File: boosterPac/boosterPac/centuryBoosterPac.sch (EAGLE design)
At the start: 5 parts, among them J1 22-05-7028-02, J2 22-05-7028-02, Q1 BSS123

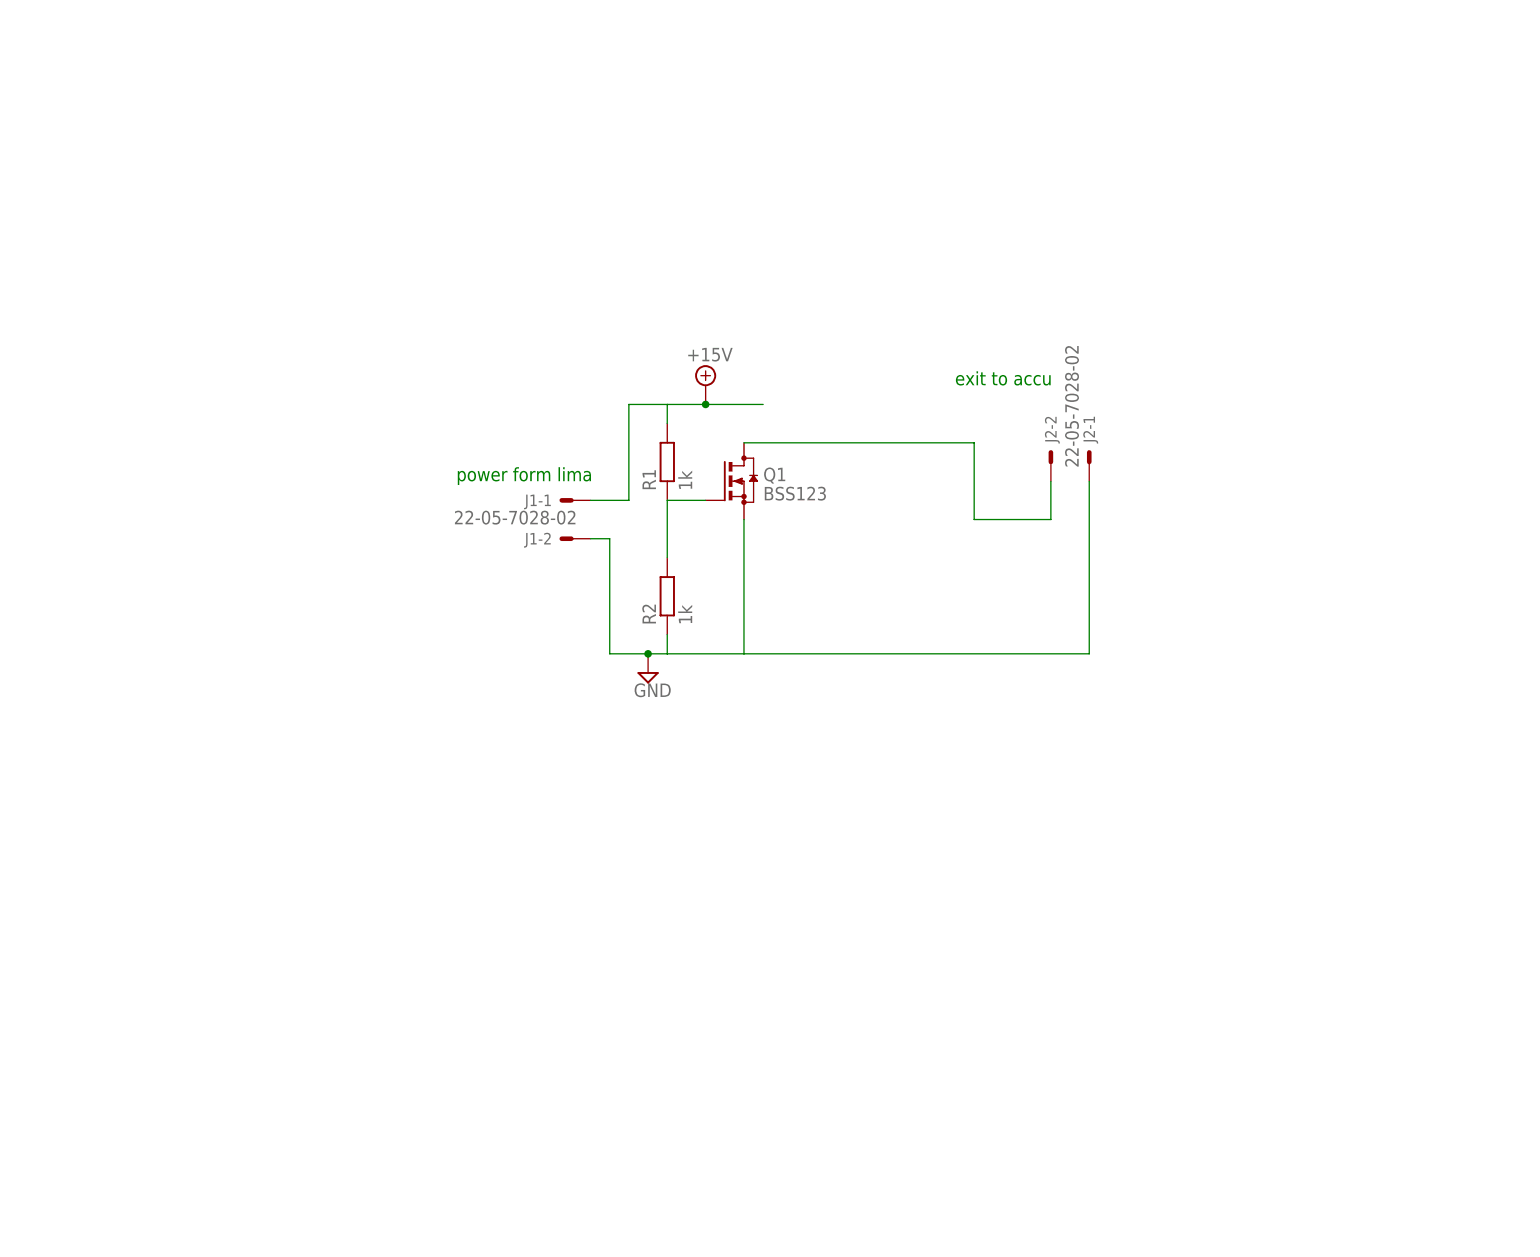
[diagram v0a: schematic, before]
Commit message: reg save
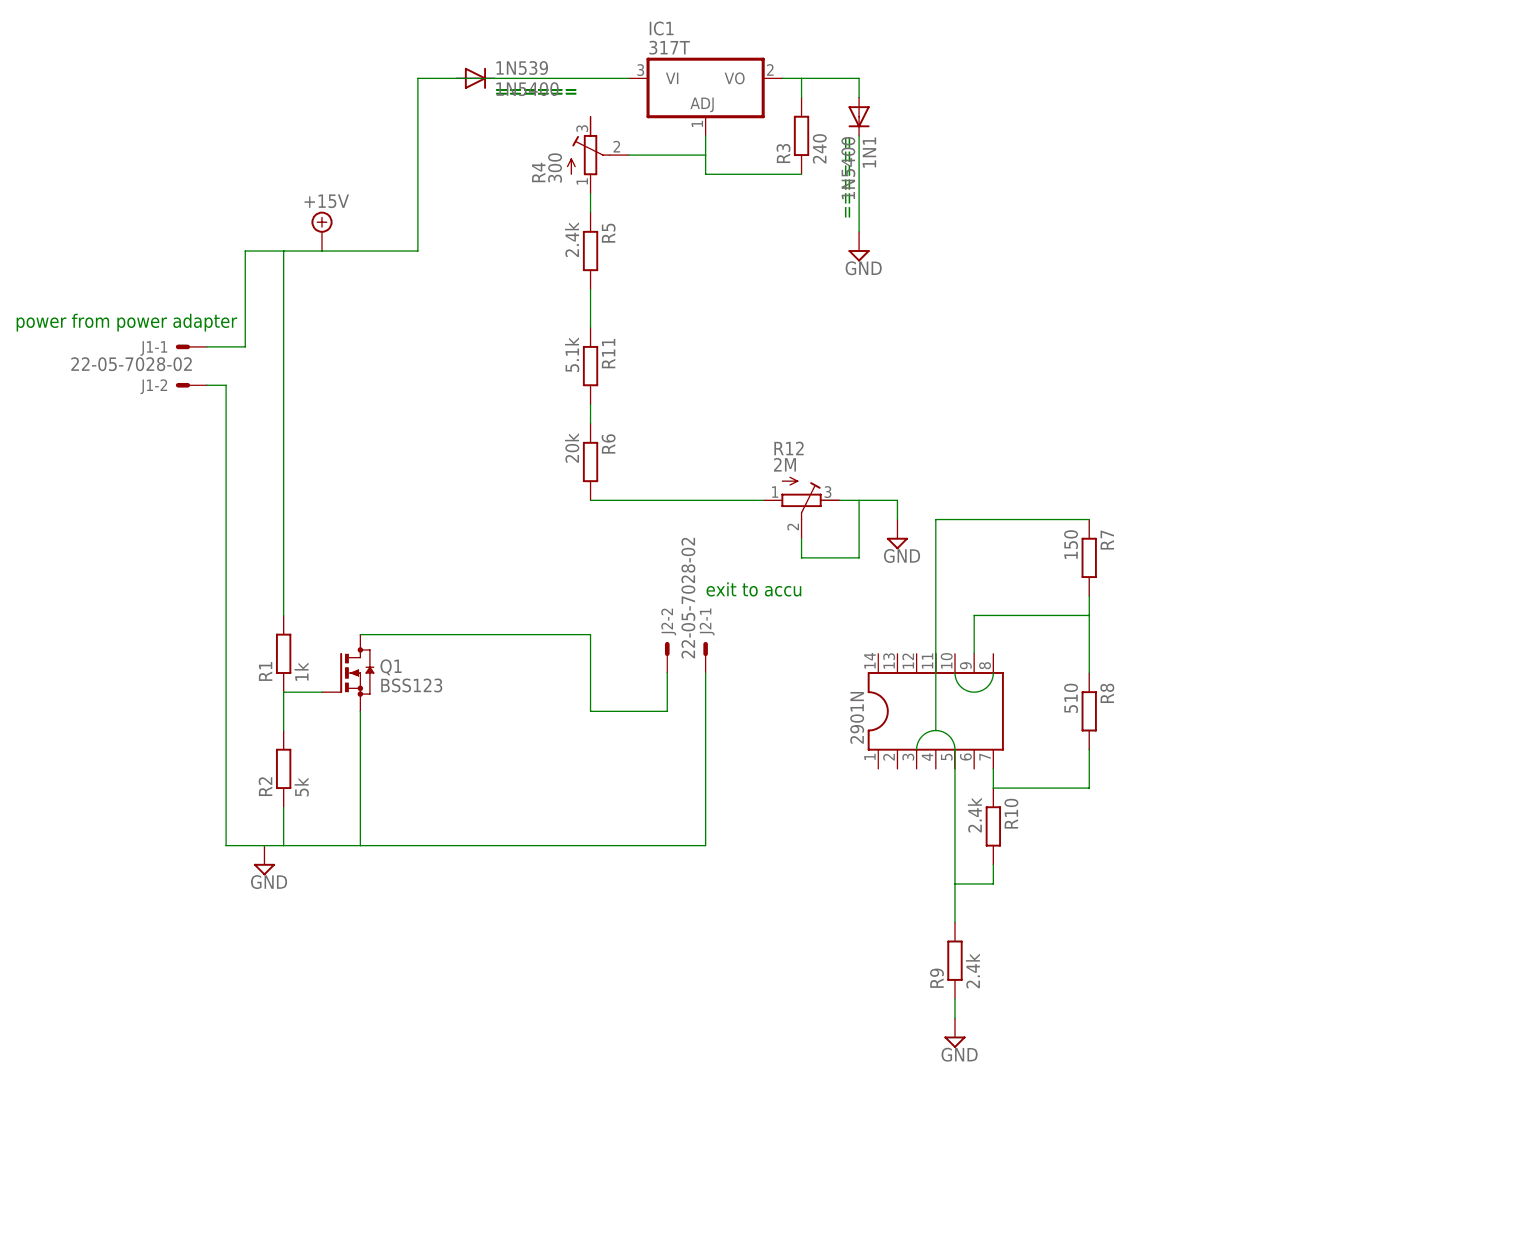
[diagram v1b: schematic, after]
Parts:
- added 1N1, 1N539: 1N5400, diode:1N5400
- added 2901N: (no value), ic-package:DIL14
- added IC1: 317T, linear:317T
- added R10, R5, R9: 2.4k, resistor:R-EU_0309/10
- added R11: 5.1k, resistor:R-EU_0309/10
- added R12: 2M, rcl:R-TRIMM3202
- added R3: 240, resistor:R-EU_0309/10
- added R4: 300, rcl:R-TRIMM3202
- added R6: 20k, resistor:R-EU_0309/10
- added R7: 150, resistor:R-EU_0309/10
- added R8: 510, resistor:R-EU_0309/10
- R2: value 1k -> 5k
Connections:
- new net N$10: 2901N.7, R10.1, R8.2
- new net N$11: 2901N.9, R7.2, R8.1
- new net N$12: 2901N.11, R7.1
- new net N$2: 1N1.A, IC1.VO, R3.2
- new net N$3: R4.A, R5.1
- new net N$4: IC1.ADJ, R3.1, R4.S
- new net N$5: R11.1, R5.2
- new net N$6: R11.2, R6.1
- new net N$7: R12.A, R6.2
- new net N$8: R12.S
- new net N$9: R10.2, R9.2
- net +15V: now also 1N539.A, 1N539.C, IC1.VI
- net GND: now also 1N1.C, R12.E, R9.1
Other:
- note added: "======"
- note added: "power from power adapter"
- note removed: "power form lima"
- moved on the sheet: J1-1, J1-2, J2-1, J2-2, Q1, R1, R2

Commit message: reg save
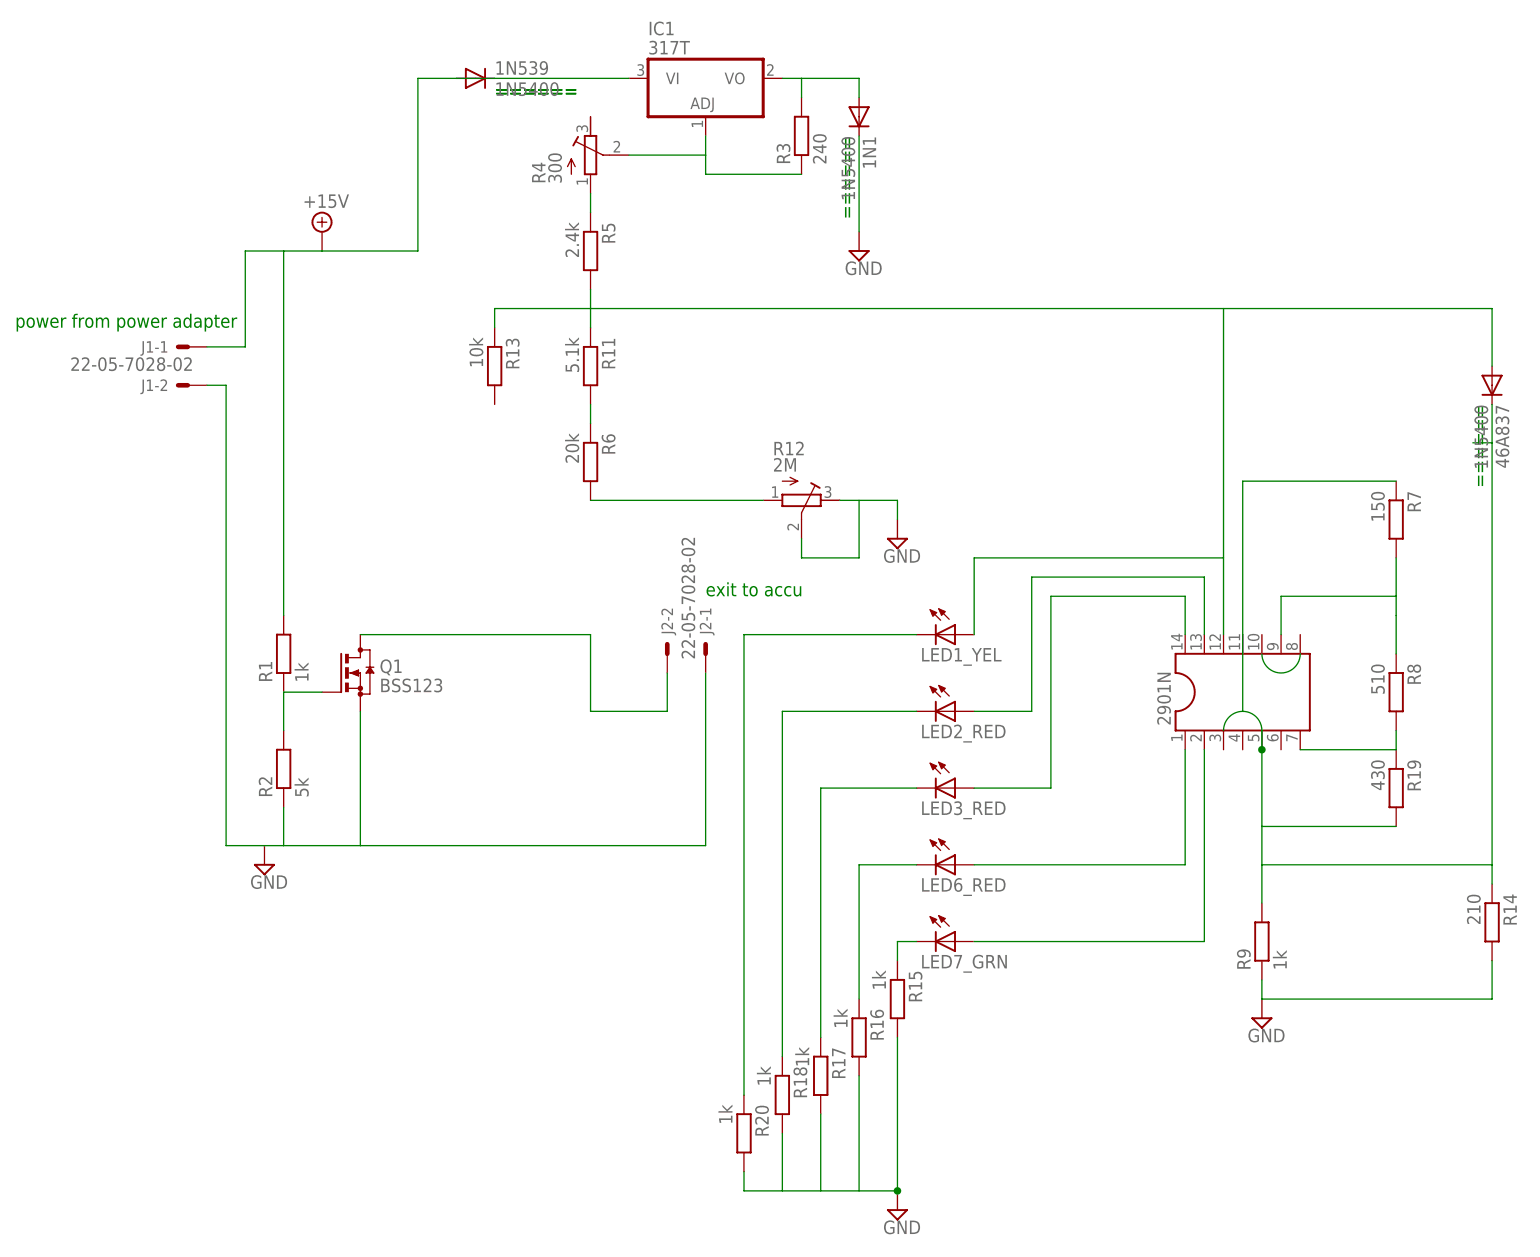
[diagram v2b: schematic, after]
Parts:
- removed R10: 2.4k, resistor:R-EU_0309/10
- added 46A837: 1N5400, diode:1N5400
- added LED1_YEL, LED2_RED, LED3_RED, LED6_RED, LED7_GRN: (no value), led:LED
- added R13: 10k, resistor:R-EU_0309/10
- added R14: 210, resistor:R-EU_0309/10
- added R15, R16, R17, R18, R20: 1k, resistor:R-EU_0309/10
- added R19: 430, resistor:R-EU_0309/10
- R9: value 2.4k -> 1k
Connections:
- removed net N$10: 2901N.7, R10.1, R8.2
- new net N$14: 2901N.5, 46A837.C, R14.1, R19.2, R9.2
- new net N$15: LED6_RED.C, R16.1
- new net N$16: LED3_RED.C, R17.1
- new net N$17: LED2_RED.C, R18.1
- new net N$18: LED1_YEL.C, R20.1
- new net N$20: R18.2
- new net N$21: R17.2
- new net N$22: R16.2
- new net N$23: 2901N.13, LED2_RED.A
- new net N$24: 2901N.14, LED3_RED.A
- new net N$25: 2901N.1, LED6_RED.A
- new net N$26: 2901N.2, LED7_GRN.A
- new net N$27: 2901N.7, R19.1, R8.2
- net GND: now also R14.2, R15.2, R20.2
- net N$5: now also 2901N.12, 46A837.A, LED1_YEL.A, R13.1
- net N$9: now also LED7_GRN.C, R15.1; no longer R10.2, R9.2
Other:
- moved on the sheet: 2901N, R7, R8, R9
